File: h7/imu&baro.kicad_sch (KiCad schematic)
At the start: 3 parts, among them U301 ICM-42688-P, U302 ICM-42688-P, U303 DPS310XTSA1

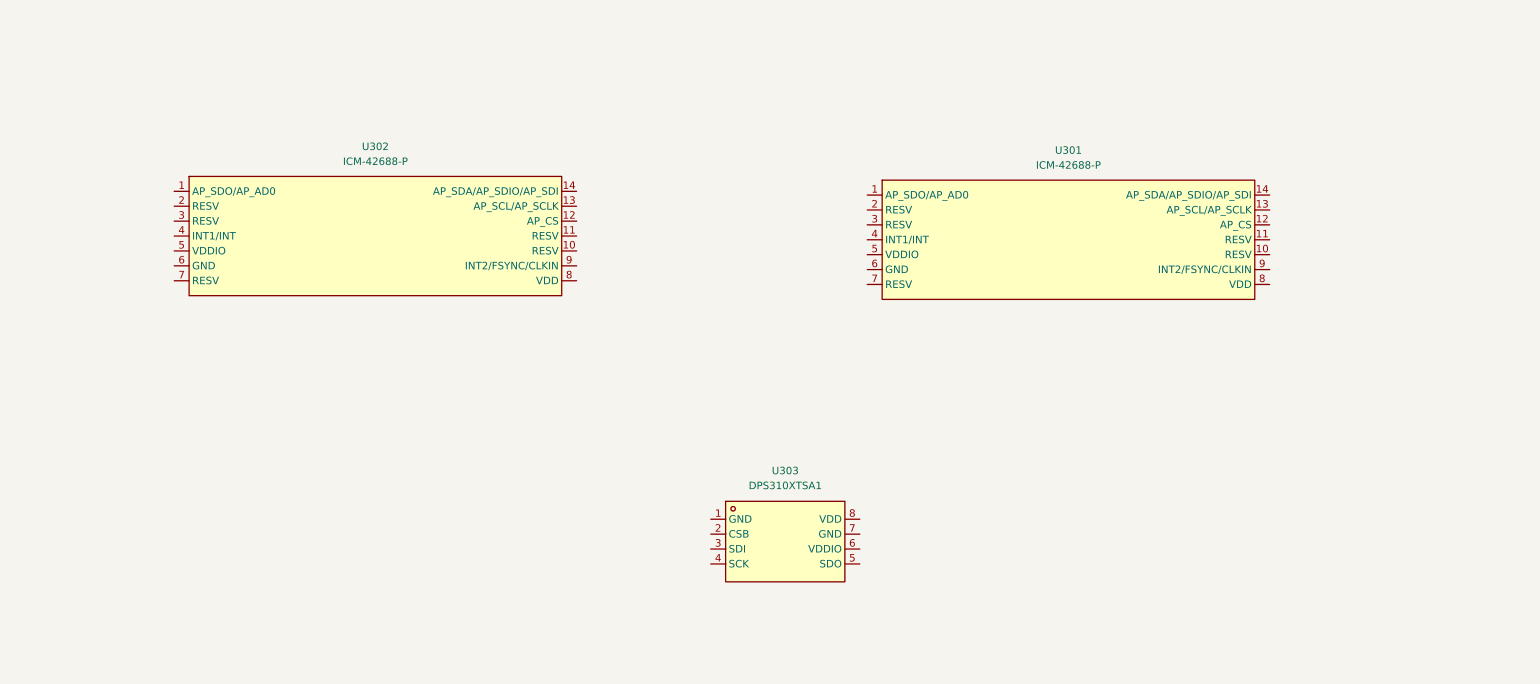
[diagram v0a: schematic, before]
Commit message: todays progresss
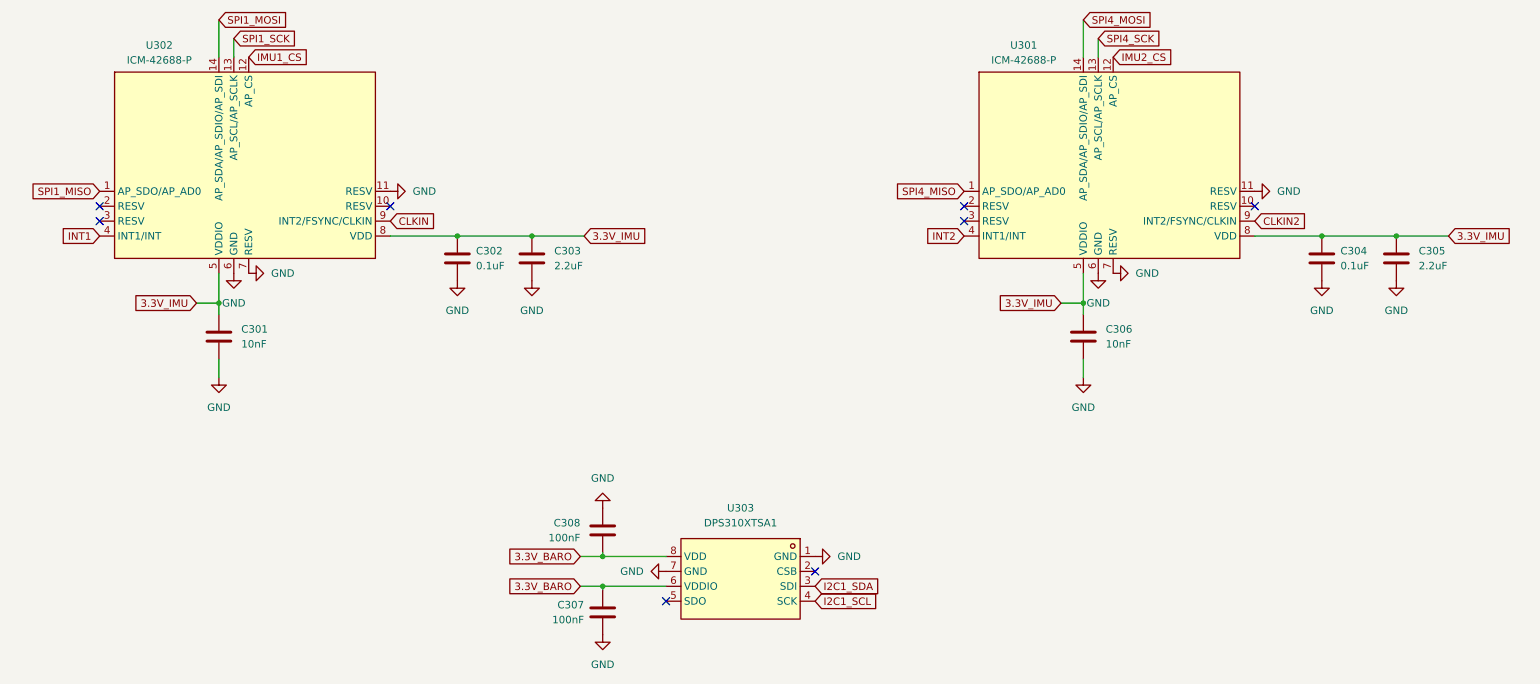
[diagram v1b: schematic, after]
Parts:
- added C301, C306: 10nF, PCM_Capacitor_SMD_AKL:C_0402_1005Metric, symbol PCM_Capacitor_AKL:C_0402
- added C302, C304: 0.1uF, PCM_Capacitor_SMD_AKL:C_0402_1005Metric, symbol PCM_Capacitor_AKL:C_0402
- added C303, C305: 2.2uF, PCM_Capacitor_SMD_AKL:C_0402_1005Metric, symbol PCM_Capacitor_AKL:C_0402
- added C307, C308: 100nF, PCM_Capacitor_SMD_AKL:C_0402_1005Metric, symbol PCM_Capacitor_AKL:C_0402
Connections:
- net SPI4_MISO: now reaches U301.1 (AP_SDO/AP_AD0)
- net GND: now reaches U301.11 (RESV)
- net GND: now also U301.6 (GND), U301.7 (RESV), U302.11 (RESV), U302.6 (GND), U302.7 (RESV), U303.1 (GND), U303.7 (GND), C301.2, C302.2, C303.2, C304.2, C305.2, C306.2, C307.2, C308.2
- net IMU2_CS: now reaches U301.12 (AP_CS)
- net SPI4_SCK: now reaches U301.13 (AP_SCL/AP_SCLK)
- net SPI4_MOSI: now reaches U301.14 (AP_SDA/AP_SDIO/AP_SDI)
- net INT2: now reaches U301.4 (INT1/INT)
- net 3.3V_IMU: now reaches U301.5 (VDDIO)
- net 3.3V_IMU: now also U301.8 (VDD), U302.5 (VDDIO), U302.8 (VDD), C301.1, C302.1, C303.1, C304.1, C305.1, C306.1
- net CLKIN2: now reaches U301.9 (INT2/FSYNC/CLKIN)
- net I2C1_SDA: now reaches U303.3 (SDI)
- net I2C1_SCL: now reaches U303.4 (SCK)
- net 3.3V_BARO: now reaches U303.6 (VDDIO)
- net 3.3V_BARO: now also U303.8 (VDD), C307.1, C308.1
- net SPI1_MISO: now reaches U302.1 (AP_SDO/AP_AD0)
- net IMU1_CS: now reaches U302.12 (AP_CS)
- net SPI1_SCK: now reaches U302.13 (AP_SCL/AP_SCLK)
- net SPI1_MOSI: now reaches U302.14 (AP_SDA/AP_SDIO/AP_SDI)
- net INT1: now reaches U302.4 (INT1/INT)
- net CLKIN: now reaches U302.9 (INT2/FSYNC/CLKIN)
- no-connect marks 0 -> 8
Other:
- moved on the sheet: U302, U303
